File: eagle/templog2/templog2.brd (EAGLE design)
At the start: 30 x 65 mm, 75 parts, among them IC1 MCP170312MB, IC3 FE1.1S, J2 CORTEX_DEBUG_PTH, J3 POWER_JACKPTH_BREAD, J4 POWER_JACKPTH_BREAD, Q4 200mA/50V, U1 ATSAMD21G-A, U3 MP2307, X2 ZX62D-B-5PA8, Y1 32.768kHz, Y2 12MHz

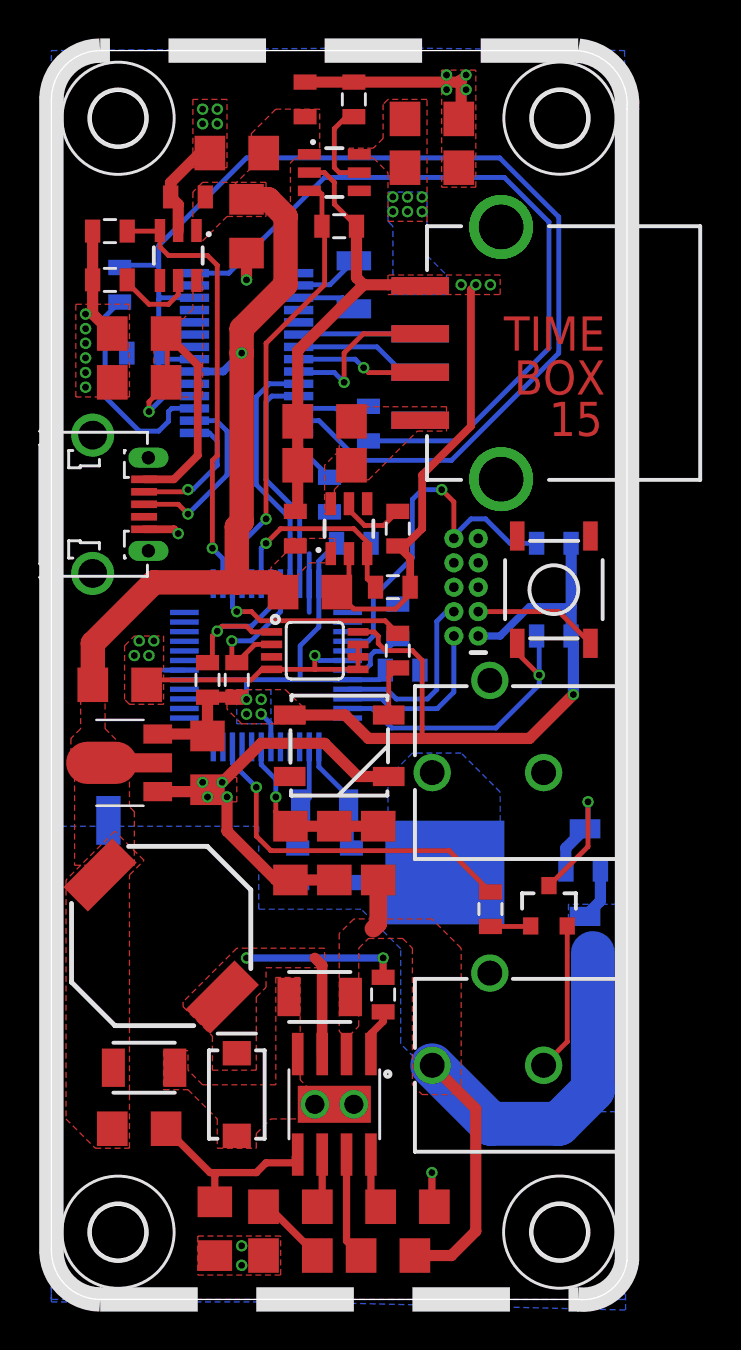
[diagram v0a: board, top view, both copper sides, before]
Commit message: new PCB files (batteryholder, templog2, ...)
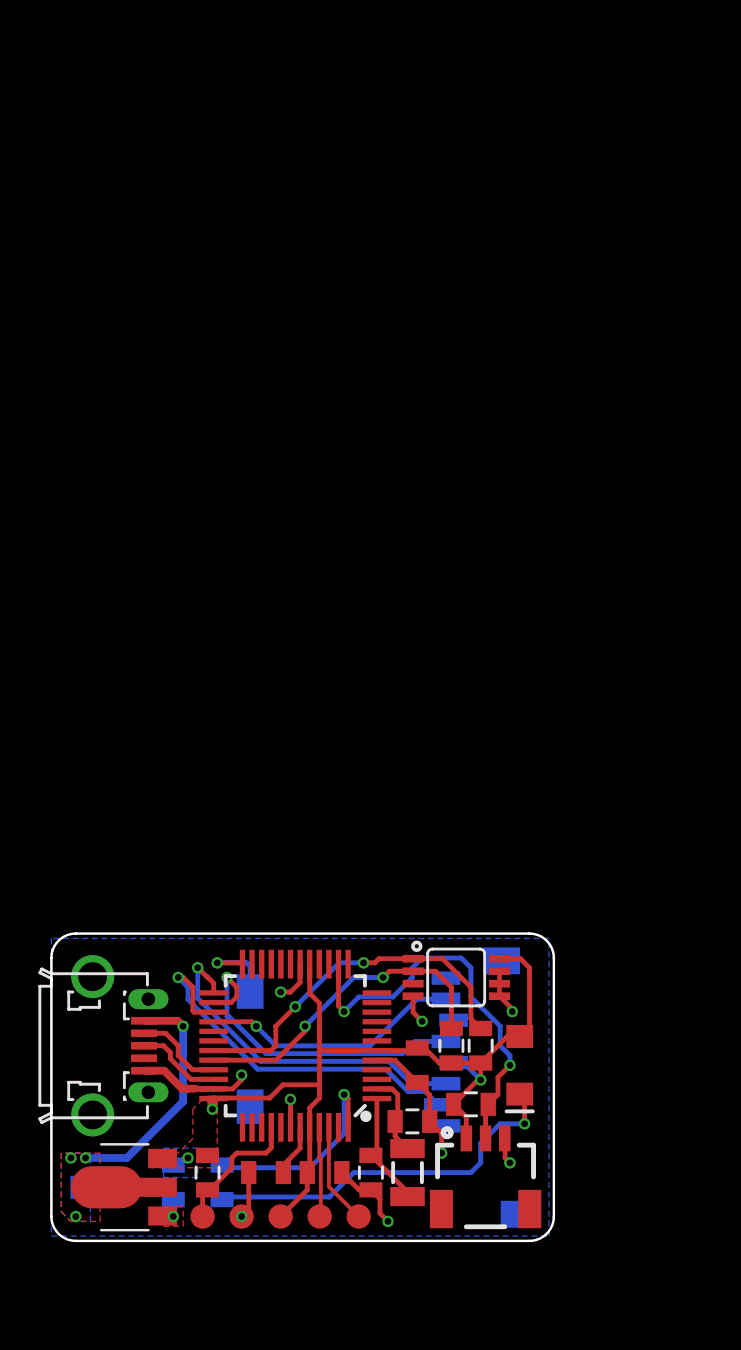
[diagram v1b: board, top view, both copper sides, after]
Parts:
- removed AP1, AP2, AP2553: MCP4725, SparkFun-IC-Conversion:SOT23-6
- removed C1, C11, C17, C22, C9: 0.1uF, SparkFun-Capacitors:0805
- removed C10, C21: 10uF, SparkFun-Capacitors:1206
- removed C12, C18, C23: 1.0uF, SparkFun-Capacitors:1206
- removed C13: 10nF, SparkFun-Capacitors:0805
- removed C14: 3.9nF, SparkFun-Capacitors:1206
- removed C15: 0.1uF, SparkFun-Capacitors:1206
- removed C16: 22uF / 6.3V, SparkFun-Capacitors:1210
- removed C19: 10uF / 25V, SparkFun-Capacitors:1210
- removed C20, C24: 120uF, SparkFun-Capacitors:1206
- removed C25: 1.0uF, SparkFun-Capacitors:0805
- removed C28, C29: 10uF, SparkFun-Capacitors:0805
- removed D2: (no value), SparkFun-LED:WS2812B
- removed H1, H2, H3, H4: MOUNT-HOLE2.8, holes:2,8
- removed IC3: FE1.1S, FE1.1S:SOP64P600X175-28N
- removed J3, J4: POWER_JACKPTH_BREAD, SparkFun-Connectors:POWER_JACK_PTH_BREAD
- removed L2: 10uH / 4A, SparkFun-Passives:SRU1038
- removed Q3: (no value), transistor-fet:TO252
- removed Q4: 200mA/50V, SparkFun-DiscreteSemi:SOT23-3
- removed R1: 6.8k, SparkFun-Resistors:1206
- removed R2: 10k / 1%, SparkFun-Resistors:1206
- removed R24: 100K, SparkFun-Resistors:1206
- removed R3: 44k / 1%, SparkFun-Resistors:1206
- removed R4: 10k, SparkFun-Resistors:0805
- removed R5, RRST1: (no value), SparkFun-Passives:0805
- removed R6: 1k, SparkFun-Resistors:0805
- removed R7, R_MOSFET_USB3, R_MOSFET_USB4, R_MOSFET_USB6: 10k, SparkFun-Passives:0805
- removed REXT: 2.7k / 1%, SparkFun-Passives:0805
- removed R_LED: 470, SparkFun-Resistors:0805
- removed R_MOSFET_USB1, R_MOSFET_USB2, R_MOSFET_USB5: ? (1%), SparkFun-Passives:0805
- removed S1: TAC_SWITCHSMD, SparkFun-Retired:TACTILE-SWITCH-SMD
- removed SH2: SHORT-HT5, shorts:SHORT_TOP-50
- removed U3: MP2307, SparkFun-AnalogIC:SO08
- removed USB_1, USB_2: USB_A_SMT_FEMALE, SparkFun-Connectors:USB-A-S-SILK-FEMALE
- removed VD1: 10k, SparkFun-Passives:1206
- removed VD2: 6.2k, SparkFun-Passives:1206
- removed Y1: 32.768kHz, SparkFun-FreqCtrl:CRYSTAL-SMD-3.2X1.5MM
- added RRST: 10k, SparkFun-Passives:0805
- added R_I2C_3: 4.7k, SparkFun-Passives:0805
- added R_I2C_4: (no value), SparkFun-Passives:0805
- added TP1, TP2, TP3, TP4, TP5: TPB1,27, testpad:B1,27
- added U$1: MICROSD, adafruit:MICROSD
- C2: value 120uF -> 0.1uF; device SparkFun-Capacitors:1206 -> SparkFun-Capacitors:0805
- C3: value 10uF -> 0.1uF; device SparkFun-Capacitors:1206 -> SparkFun-Capacitors:0805
- C6: value 0.1uF -> 1.0uF; device SparkFun-Capacitors:1206 -> SparkFun-Capacitors:0805
- C7, C8: device SparkFun-Capacitors:1206 -> SparkFun-Capacitors:0805
- D1: value 3A/40V/500mV -> (none); device SparkFun-DiscreteSemi:SMA-DIODE -> SparkFun-LED:LED-1206
- J2: value CORTEX_DEBUG_PTH -> (none); device SparkFun-Connectors:2X5-PTH-1.27MM -> SparkFun-Connectors:1X03-1MM-RA
- Y2: value 12MHz -> 32.768kHz; device SparkFun-FreqCtrl:CRYSTAL-SMD-3.2X1.5MM -> samd21-temp:CRYSTAL-SMD-3.2X1.5MM
- moved C3 48.4 mm to (19.1, 12.2), turned to 90 degrees
- moved Y2 46.3 mm to (18.5, 6.60), flipped to the top, turned to 270 degrees
- moved C2 39.1 mm to (14.2, 6.60), turned to 180 degrees
- moved J2 28.7 mm to (22.6, 8.38), turned to 0 degrees
- moved X2 28.2 mm to (0.00, 13.2)
- moved C7 26.2 mm to (2.29, 5.84), flipped to the bottom, turned to 180 degrees
- moved R_I2C_2 23.8 mm to (22.4, 13.2)
- moved IC1 22.1 mm to (3.81, 5.84)
- moved R_I2C_1 22.1 mm to (20.8, 13.2)
- moved C8 21.9 mm to (6.35, 6.10), flipped to the bottom
- moved U1 19.9 mm to (12.7, 13.2), flipped to the top, turned to 180 degrees
- moved MCP9808 18.5 mm to (21.1, 16.8)
- moved C6 16.7 mm to (11.2, 6.60), turned to 180 degrees
- moved C4 16.0 mm to (16.6, 6.60), flipped to the top
- moved D1 14.8 mm to (24.4, 12.2), turned to 270 degrees
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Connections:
- removed net BATT_VCC: C19.2, J4.PWR, Q3.2, R24.1, R4.1, U3.2, VD1.2
- removed net BTN: R5.2, S1.4, U1.47
- removed net CAM_EN: R6.1, U1.10
- removed net CAM_OUT: J3.PWR, Q3.3
- removed net CONV_5V: C16.2, L2.1, R3.2
- removed net GNDA: C15.1, C16.1, C19.1, D1.A, R1.2, R2.2, SH2.1, U3.4, U3.BTM, U3.P$1
- removed net N$10: AP1.5, R_MOSFET_USB2.2
- removed net N$11: AP2.5, R_MOSFET_USB5.2
- removed net N$15: IC3.17, R7.1
- removed net N$2: Q4.1, R6.2
- removed net N$23: IC3.3, Y2.P$1
- removed net N$24: IC3.2, Y2.P$2
- removed net N$25: C15.2, U3.8
- removed net N$26: C13.2, D1.C, L2.2, U3.3
- removed net N$27: C13.1, U3.1
- removed net N$28: C14.1, R1.1
- removed net N$29: C14.2, U3.6
- removed net N$3: Q3.1, Q4.3, R4.2
- removed net N$30: R2.1, R3.1, U3.5
- removed net N$31: IC3.14, REXT.2
- removed net N$7: D2.4, R_LED.2
- removed net N$9: AP2553.5, R_MOSFET_USB1.2
- removed net PB_BUCK_EN: R24.2, U3.7
- removed net UC_DM: IC3.10, U1.33
- removed net UC_DP: IC3.11, U1.34
- removed net USB0_EN: AP2.3, R_MOSFET_USB6.2, U1.26
- removed net USB1_EN: AP2553.3, R_MOSFET_USB3.2, U1.30
- removed net USB1_OUT: AP2553.6, C12.2, C2.2, USB_1.VBUS
- removed net USB2_EN: AP1.3, R_MOSFET_USB4.2, U1.28
- removed net USB2_OUT: AP1.6, C18.2, C20.2, USB_2.VBUS
- removed net USB_1_DM: IC3.8, USB_1.D-
- removed net USB_1_DP: IC3.9, USB_1.D+
- removed net USB_2_DM: IC3.6, USB_2.D-
- removed net USB_2_DP: IC3.7, USB_2.D+
- removed net USB_3_DM: IC3.4
- removed net USB_3_DP: IC3.5
- removed net VCC_5V: AP1.1, AP2.1, AP2553.1, C10.1, C11.1, C17.1, C21.1, C22.1, C3.1, C7.1, IC1.2@1, IC3.20
- removed net VD_18: C28.1, IC3.12, IC3.28
- removed net VD_33: C29.2, IC3.13, IC3.19, IC3.21, IC3.26, R7.2
- removed net VD_INT: C6.1, U1.7, VD1.1, VD2.2
- new net CD: U$1.CD1, U1.24
- new net CS: U$1.2, U1.27
- new net EXT_SENSOR: J2.2, R_I2C_3.1, U1.14
- new net MISO: U$1.7, U1.28
- new net MOSI: U$1.3, U1.25
- new net N$1: C6.1, U1.43
- new net SCK: U$1.5, U1.26
- net GND: now also C3.1, TP5.TP, U$1.6, U$1.MT1, U$1.MT2, U1.5; no longer AP1.2, AP2.2, AP2553.2, C1.2, C10.2, C11.2, C12.1, C17.2, C18.1, C20.1, C21.2, C22.2, C23.1, C24.1, C25.1, C28.2, C29.1, C3.2, C9.2, D2.3, IC3.1, J2.5, J3.GND, J4.GND, Q4.2, REXT.1, R_MOSFET_USB1.1, R_MOSFET_USB2.1, R_MOSFET_USB3.1, R_MOSFET_USB4.1, R_MOSFET_USB5.1, R_MOSFET_USB6.1, S1.2, SH2.2, USB_1.GND, USB_2.GND, VD2.1
- net LED: now also R_I2C_4.2, U1.48; no longer R_LED.1, U1.27
- net MICRO_DM: now also U1.33; no longer IC3.15
- net MICRO_DP: now also U1.34; no longer IC3.16
- net MICRO_VBUS: now also C7.1, IC1.2@1; no longer AP2.6, C23.2, C24.2, IC3.18
- net N$32: now also Y2.P$1; no longer Y1.P$1
- net N$5: now also D1.C, R_I2C_4.1; no longer C25.2, U1.43
- net N$8: now also Y2.P$2; no longer Y1.P$2
- net RESET: now also RRST.1, TP3.TP; no longer J2.10, RRST1.1
- net SWDCLK: now also TP2.TP; no longer J2.4
- net SWDIO: now also TP1.TP; no longer J2.2
- net VCC: now also C2.2, C3.2, D1.A, RRST.2, R_I2C_3.2, TP4.TP, U$1.4; no longer C1.1, C9.1, D2.1, R5.1, RRST1.2
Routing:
- net GND: track 128.3 -> 28.3 mm, vias 28 -> 10
- net VD_33: track 62.9 -> 0.00 mm
- net VD_18: track 43.8 -> 0.00 mm
- net VCC_5V: track 38.9 -> 0.00 mm, vias 1 -> 0
- net BATT_VCC: track 36.1 -> 0.00 mm
- net USB0_EN: track 22.9 -> 0.00 mm, vias 1 -> 0
- net USB2_EN: track 22.8 -> 0.00 mm, vias 1 -> 0
- net VCC: track 65.7 -> 44.5 mm, vias 5 -> 3
- net EXT_SENSOR: track 0.00 -> 21.1 mm, vias 0 -> 2
- net CS: track 0.00 -> 20.0 mm, vias 0 -> 1
- net CAM_EN: track 18.6 -> 0.00 mm, vias 1 -> 0
- net MOSI: track 0.00 -> 18.0 mm, vias 0 -> 1
- net SCK: track 0.00 -> 17.0 mm, vias 0 -> 1
- net N$5: track 3.55 -> 19.6 mm, vias 0 -> 1
- net BTN: track 16.0 -> 0.00 mm, vias 1 -> 0
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- added copper zone on layer 16, net MICRO_VBUS
- removed copper zone on layer 1, net BATT_VCC
- removed copper zone on layer 16, net BATT_VCC
- removed copper zone on layer 16, net CAM_OUT
- removed copper zone on layer 1, net CONV_5V
- removed copper zone on layer 1, net GNDA
- removed copper zone on layer 16, net GNDA
- removed copper zone on layer 1, net N$26
- removed copper zone on layer 1, net USB1_OUT
- removed copper zone on layer 1, net USB2_OUT
- removed copper zone on layer 16, net USB2_OUT
- removed copper zone on layer 1, net VCC_5V
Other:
- board size 30 x 65 mm -> 26.2 x 16 mm
- board text added: "TEMPlog2"
- board text removed: "15"
- board text removed: "BOX"
- board text removed: "IN"
- board text removed: "OUT"
- board text removed: "TIME"
